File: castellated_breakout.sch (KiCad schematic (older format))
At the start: 3 parts, among them J1 Conn_01x14_Female, J2 Conn_01x14_Female, U1 STM32_7x4_Castellated

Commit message: board layout + route
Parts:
- J1, J2: footprint (none) -> Connector_PinSocket_2.54mm:PinSocket_1x14_P2.54mm_Vertical
- U1: footprint (none) -> castellated_breakout:7x4_Castellated
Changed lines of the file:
@@
 F 0 "U1" H 5825 4265 50  0000 C CNN
 F 1 "STM32_7x4_Castellated" H 5825 4174 50  0000 C CNN
-F 2 "" H 6050 3550 50  0001 C CNN
+F 2 "castellated_breakout:7x4_Castellated" H 6050 3550 50  0001 C CNN
 F 3 "" H 6050 3550 50  0001 C CNN
 	1    6050 3550
@@
 F 0 "J1" H 4492 2925 50  0000 C CNN
 F 1 "Conn_01x14_Female" H 4492 3016 50  0000 C CNN
-F 2 "" H 4600 3850 50  0001 C CNN
+F 2 "Connector_PinSocket_2.54mm:PinSocket_1x14_P2.54mm_Vertical" H 4600 3850 50  0001 C CNN
 F 3 "~" H 4600 3850 50  0001 C CNN
 	1    4600 3850
@@
 F 0 "J2" H 7078 3726 50  0000 L CNN
 F 1 "Conn_01x14_Female" H 7078 3635 50  0000 L CNN
-F 2 "" H 7050 3750 50  0001 C CNN
+F 2 "Connector_PinSocket_2.54mm:PinSocket_1x14_P2.54mm_Vertical" H 7050 3750 50  0001 C CNN
 F 3 "~" H 7050 3750 50  0001 C CNN
 	1    7050 3750

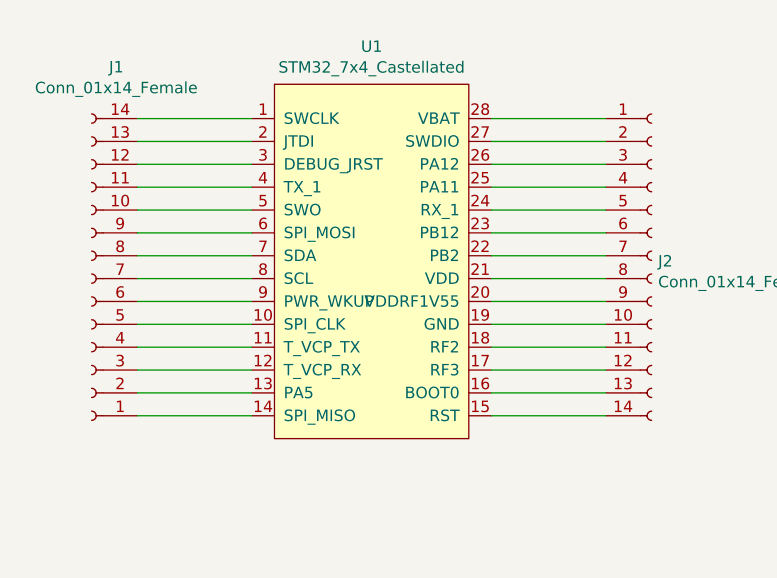
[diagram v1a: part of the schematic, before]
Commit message: v2 voltera, v1 pcbway
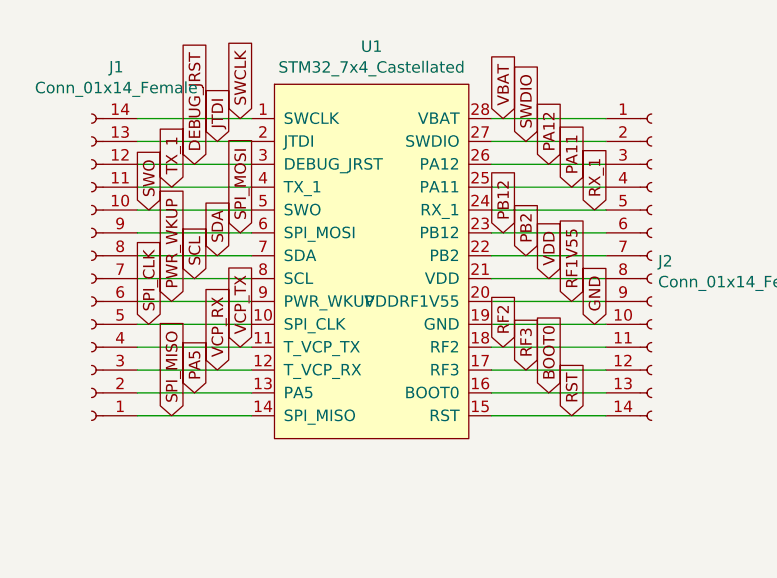
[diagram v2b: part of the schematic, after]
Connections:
- net SWCLK: now reaches J1.14 (Pin_14), U1.1 (SWCLK)
- net SPI_CLK: now reaches J1.5 (Pin_5), U1.10 (SPI_CLK)
- net VCP_TX: now reaches J1.4 (Pin_4), U1.11 (T_VCP_TX)
- net VCP_RX: now reaches J1.3 (Pin_3), U1.12 (T_VCP_RX)
- net PA5: now reaches J1.2 (Pin_2), U1.13 (PA5)
- net SPI_MISO: now reaches J1.1 (Pin_1), U1.14 (SPI_MISO)
- net RST: now reaches J2.14 (Pin_14), U1.15 (RST)
- net BOOT0: now reaches J2.13 (Pin_13), U1.16 (BOOT0)
- net RF3: now reaches J2.12 (Pin_12), U1.17 (RF3)
- net RF2: now reaches J2.11 (Pin_11), U1.18 (RF2)
- net GND: now reaches J2.10 (Pin_10), U1.19 (GND)
- net JTDI: now reaches J1.13 (Pin_13), U1.2 (JTDI)
- net RF1V55: now reaches J2.9 (Pin_9), U1.20 (VDDRF1V55)
- net VDD: now reaches J2.8 (Pin_8), U1.21 (VDD)
- net PB2: now reaches J2.7 (Pin_7), U1.22 (PB2)
- net PB12: now reaches J2.6 (Pin_6), U1.23 (PB12)
- net RX_1: now reaches J2.5 (Pin_5), U1.24 (RX_1)
- net PA11: now reaches J2.4 (Pin_4), U1.25 (PA11)
- net PA12: now reaches J2.3 (Pin_3), U1.26 (PA12)
- net SWDIO: now reaches J2.2 (Pin_2), U1.27 (SWDIO)
- net VBAT: now reaches J2.1 (Pin_1), U1.28 (VBAT)
- net DEBUG_JRST: now reaches J1.12 (Pin_12), U1.3 (DEBUG_JRST)
- net TX_1: now reaches J1.11 (Pin_11), U1.4 (TX_1)
- net SWO: now reaches J1.10 (Pin_10), U1.5 (SWO)
- net SPI_MOSI: now reaches J1.9 (Pin_9), U1.6 (SPI_MOSI)
- net SDA: now reaches J1.8 (Pin_8), U1.7 (SDA)
- net SCL: now reaches J1.7 (Pin_7), U1.8 (SCL)
- net PWR_WKUP: now reaches J1.6 (Pin_6), U1.9 (PWR_WKUP)
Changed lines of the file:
@@
 Wire Wire Line
 	6850 4450 6350 4450
+Text GLabel 5250 3150 1    50   Input ~ 0
+SWCLK
+Text GLabel 5150 3250 1    50   Input ~ 0
+JTDI
+Text GLabel 5050 3350 1    50   Input ~ 0
+DEBUG_JRST
+Text GLabel 4950 3450 1    50   Input ~ 0
+TX_1
+Text GLabel 4850 3550 1    50   Input ~ 0
+SWO
+Text GLabel 5250 3650 1    50   Input ~ 0
+SPI_MOSI
+Text GLabel 5150 3750 1    50   Input ~ 0
+SDA
+Text GLabel 5050 3850 1    50   Input ~ 0
+SCL
+Text GLabel 4950 3950 1    50   Input ~ 0
+PWR_WKUP
+Text GLabel 4850 4050 1    50   Input ~ 0
+SPI_CLK
+Text GLabel 5250 4150 1    50   Input ~ 0
+VCP_TX
+Text GLabel 5150 4250 1    50   Input ~ 0
+VCP_RX
+Text GLabel 5050 4350 1    50   Input ~ 0
+PA5
+Text GLabel 4950 4450 1    50   Input ~ 0
+SPI_MISO
+Text GLabel 6400 3150 1    50   Input ~ 0
+VBAT
+Text GLabel 6500 3250 1    50   Input ~ 0
+SWDIO
+Text GLabel 6600 3350 1    50   Input ~ 0
+PA12
+Text GLabel 6700 3450 1    50   Input ~ 0
+PA11
+Text GLabel 6800 3550 1    50   Input ~ 0
+RX_1
+Text GLabel 6400 3650 1    50   Input ~ 0
+PB12
+Text GLabel 6500 3750 1    50   Input ~ 0
+PB2
+Text GLabel 6600 3850 1    50   Input ~ 0
+VDD
+Text GLabel 6700 3950 1    50   Input ~ 0
+RF1V55
+Text GLabel 6800 4050 1    50   Input ~ 0
+GND
+Text GLabel 6400 4150 1    50   Input ~ 0
+RF2
+Text GLabel 6500 4250 1    50   Input ~ 0
+RF3
+Text GLabel 6600 4350 1    50   Input ~ 0
+BOOT0
+Text GLabel 6700 4450 1    50   Input ~ 0
+RST
 $EndSCHEMATC

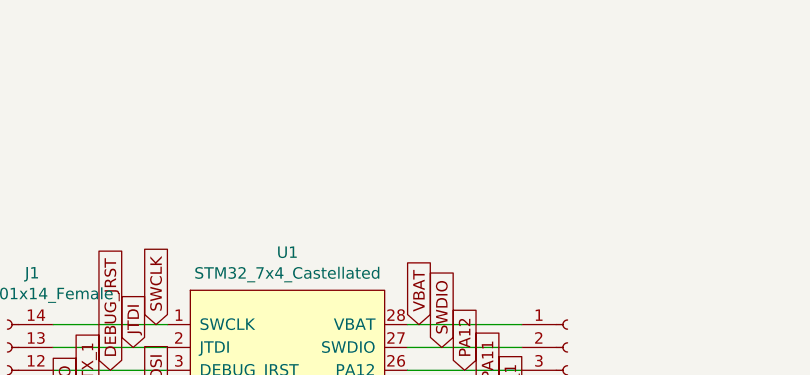
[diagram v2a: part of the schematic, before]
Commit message: v2 pcbway
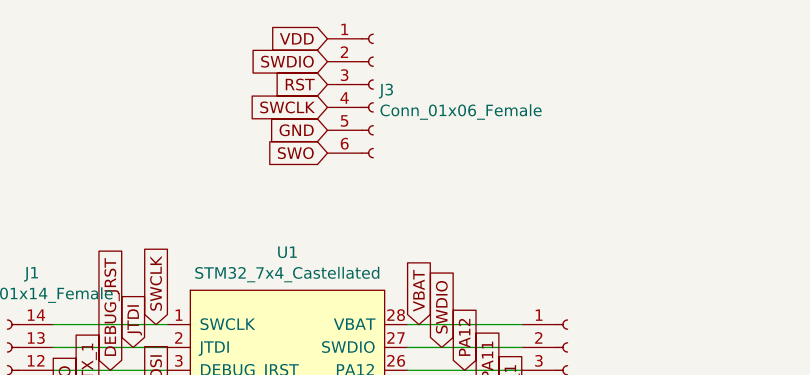
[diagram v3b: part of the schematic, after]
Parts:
- added J3: Conn_01x06_Female, Connector:Tag-Connect_TC2030-IDC-NL_2x03_P1.27mm_Vertical, symbol Connector:Conn_01x06_Female
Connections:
- net GND: now also J3.5 (Pin_5)
- net RST: now also J3.3 (Pin_3)
- net SWCLK: now also J3.4 (Pin_4)
- net SWDIO: now also J3.2 (Pin_2)
- net SWO: now also J3.6 (Pin_6)
- net VDD: now also J3.1 (Pin_1)
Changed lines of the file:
@@
 Text GLabel 6700 4450 1    50   Input ~ 0
 RST
+$Comp
+L Connector:Conn_01x06_Female J3
+U 1 1 613CFD7B
+P 6200 2100
+F 0 "J3" H 6228 2076 50  0000 L CNN
+F 1 "Conn_01x06_Female" H 6228 1985 50  0000 L CNN
+F 2 "Connector:Tag-Connect_TC2030-IDC-NL_2x03_P1.27mm_Vertical" H 6200 2100 50  0001 C CNN
+F 3 "~" H 6200 2100 50  0001 C CNN
+	1    6200 2100
+	1    0    0    -1
+$EndComp
+Text GLabel 6000 1900 0    50   Input ~ 0
+VDD
+Text GLabel 6000 2000 0    50   Input ~ 0
+SWDIO
+Text GLabel 6000 2100 0    50   Input ~ 0
+RST
+Text GLabel 6000 2200 0    50   Input ~ 0
+SWCLK
+Text GLabel 6000 2300 0    50   Input ~ 0
+GND
+Text GLabel 6000 2400 0    50   Input ~ 0
+SWO
 $EndSCHEMATC
